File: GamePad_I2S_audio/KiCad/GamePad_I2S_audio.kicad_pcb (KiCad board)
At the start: 4 copper layers, 42.2 x 47.1 mm, 48 parts, among them J1 Conn_02x17_Odd_Even

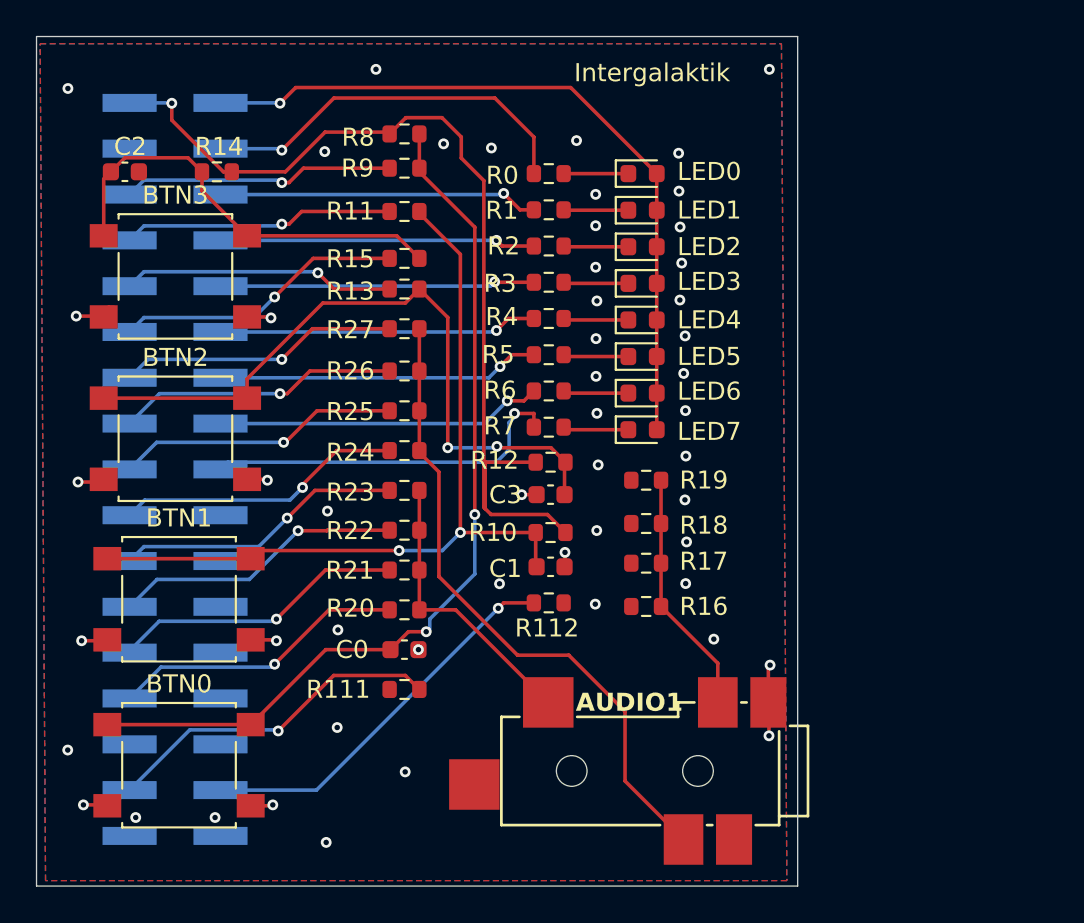
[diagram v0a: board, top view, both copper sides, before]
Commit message: initial PCB setup
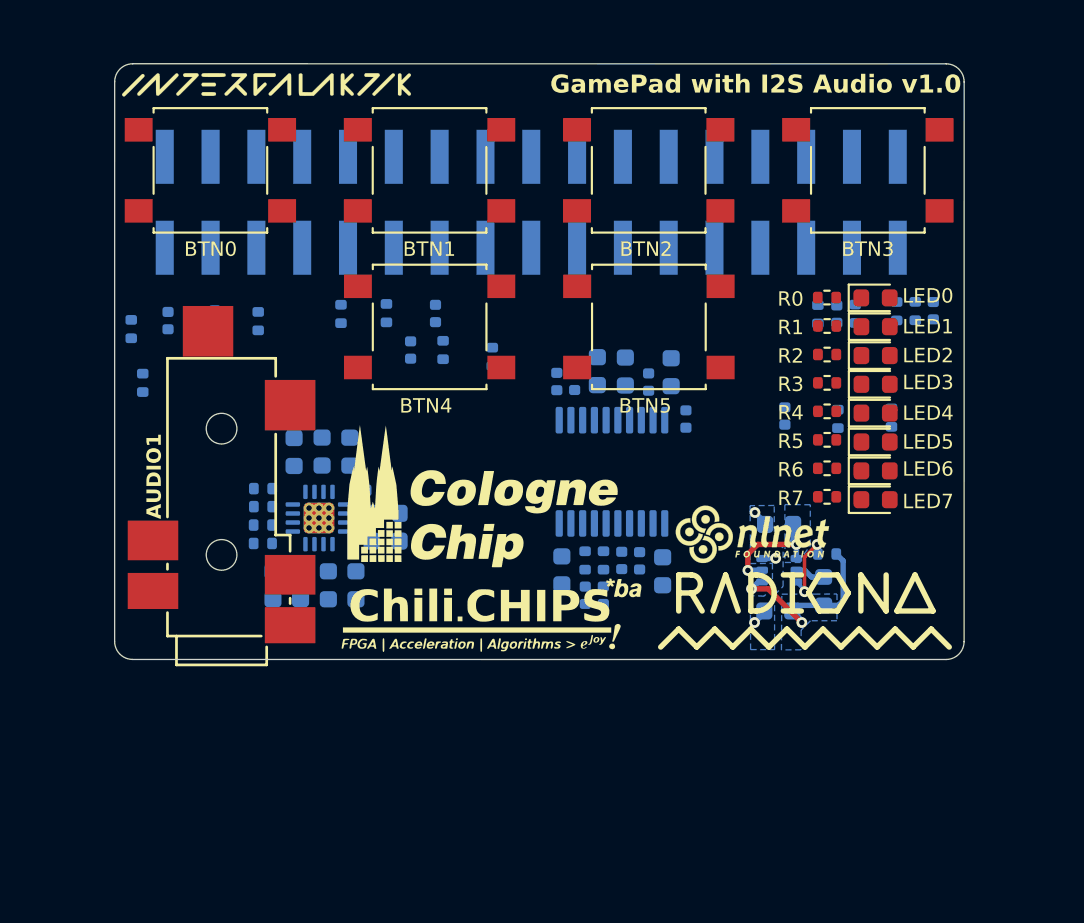
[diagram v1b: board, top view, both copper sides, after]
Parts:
- removed R21, R25: 549, Resistor_SMD:R_0603_1608Metric
- removed R22, R26: 270, Resistor_SMD:R_0603_1608Metric
- removed R23, R27: 130, Resistor_SMD:R_0603_1608Metric
- removed R24: 1.1k, Resistor_SMD:R_0603_1608Metric
- added BTN4: BTN, Button_Switch_SMD:SW_SPST_B3S-1000, F.Cu at (128.9, 68.7)
- added BTN5: BTN, Button_Switch_SMD:SW_SPST_B3S-1000, F.Cu at (141.1, 68.7)
- added C10: 100nF, Capacitor_SMD:C_0402_1005Metric, B.Cu at (141.0, 71.8)
- added C11: 10uF, Capacitor_SMD:C_0603_1608Metric, B.Cu at (138.2, 71.2)
- added C12: 2.2nF, Capacitor_SMD:C_0402_1005Metric, B.Cu at (138.5, 83.6)
- added C13: 10uF, Capacitor_SMD:C_0603_1608Metric, B.Cu at (139.7, 71.2)
- added C14: 100nF, Capacitor_SMD:C_0402_1005Metric, B.Cu at (135.9, 71.7)
- added C15: 10uF, Capacitor_SMD:C_0603_1608Metric, B.Cu at (142.3, 71.2)
- added C16: 100nF, Capacitor_SMD:C_0402_1005Metric, B.Cu at (143.1, 73.8)
- added C17: 4.7u, Capacitor_SMD:C_0603_1608Metric, B.Cu at (124.8, 83.0)
- added C18: 4.7u, Capacitor_SMD:C_0603_1608Metric, B.Cu at (123.3, 83.0)
- added C19: 4.7u, Capacitor_SMD:C_0603_1608Metric, B.Cu at (121.7, 83.0)
- added C20: 4.7u, Capacitor_SMD:C_0603_1608Metric, B.Cu at (120.2, 83.0)
- added C21: 4.7u, Capacitor_SMD:C_0603_1608Metric, B.Cu at (126.5, 80.6)
- added C22: 1u, Capacitor_SMD:C_0603_1608Metric, B.Cu at (121.4, 75.6)
- added C23: 1u, Capacitor_SMD:C_0603_1608Metric, B.Cu at (124.5, 75.6)
- added C24: 1u, Capacitor_SMD:C_0603_1608Metric, B.Cu at (122.9, 75.6)
- added C25: 100nF/10V/20%/X5R/C0402, Capacitor_SMD:C_0402_1005Metric, B.Cu at (114.4, 68.3)
- added C26: 100nF/10V/20%/X5R/C0402, Capacitor_SMD:C_0402_1005Metric, B.Cu at (148.6, 73.6)
- added C27: 10uF, Capacitor_SMD:C_0603_1608Metric, B.Cu at (148.2, 84.5)
- added C28: 10uF, Capacitor_SMD:C_0603_1608Metric, B.Cu at (148.3, 79.7)
- added C4: 10uF, Capacitor_SMD:C_0603_1608Metric, B.Cu at (141.8, 82.2)
- added C5: 10uF, Capacitor_SMD:C_0603_1608Metric, B.Cu at (136.2, 82.2)
- added C6: 100nF, Capacitor_SMD:C_0402_1005Metric, B.Cu at (136.9, 71.7)
- added C7: 2.2uF, Capacitor_SMD:C_0402_1005Metric, B.Cu at (140.5, 81.7)
- added C8: 2.2uF, Capacitor_SMD:C_0402_1005Metric, B.Cu at (139.5, 81.6)
- added C9: 2.2nF, Capacitor_SMD:C_0402_1005Metric, B.Cu at (137.5, 83.6)
- added G***: LOGO, nlnet:nlnet, F.Cu at (146.8, 80.2)
- added G***: LOGO, Cologne:cologne, F.Cu at (131.8, 78.1)
- added G***: LOGO, PCM_Intergalaktik:Intergalaktik logo, F.Cu at (119.9, 55.1)
- added G***: LOGO, ChiliChips:ChiliChipsBa, F.Cu at (132.4, 84.6)
- added IC1: PCM5100, Package_SO:TSSOP-20_4.4x6.5mm_P0.65mm, B.Cu at (139.0, 76.7)
- added IC2: PAM8908, Package_DFN_QFN:QFN-16-1EP_3x3mm_P0.5mm_EP1.7x1.7mm_ThermalVias, B.Cu at (122.8, 79.3)
- added IC3: TLV61225DC, Package_TO_SOT_SMD:SOT-363_SC-70-6, B.Cu at (148.3, 82.2)
- added L1: 80R@100M, Inductor_SMD:L_0603_1608Metric, B.Cu at (126.5, 79.0)
- added L2: 4.7uH, Inductor_SMD:L_0603_1608Metric, B.Cu at (150.7, 83.3)
- added R30: 470, Resistor_SMD:R_0402_1005Metric, B.Cu at (138.5, 81.6)
- added R31: 470, Resistor_SMD:R_0402_1005Metric, B.Cu at (137.5, 81.6)
- added R32: 33K, Resistor_SMD:R_0402_1005Metric, B.Cu at (125.9, 77.8)
- added R33: 330, Resistor_SMD:R_0402_1005Metric, B.Cu at (119.7, 78.7)
- added R34: 33K, Resistor_SMD:R_0402_1005Metric, B.Cu at (119.7, 77.7)
- added R35: 330, Resistor_SMD:R_0402_1005Metric, B.Cu at (119.7, 79.7)
- added R36: 33K, Resistor_SMD:R_0402_1005Metric, B.Cu at (119.7, 80.7)
- added radiona: radiona, radiona:radiona, F.Cu at (149.7, 83.5)
- C0, C1, C2, C3: footprint Capacitor_SMD:C_0603_1608Metric -> Capacitor_SMD:C_0402_1005Metric; moved to B.Cu
- R0, R1, R2, R3, R4, R5, R6, R7: footprint Resistor_SMD:R_0603_1608Metric -> Resistor_SMD:R_0402_1005Metric
- R10, R11, R111, R112, R12, R13, R14, R15, R8, R9: footprint Resistor_SMD:R_0603_1608Metric -> Resistor_SMD:R_0402_1005Metric; moved to B.Cu
- R16: value 1.1k -> 22R/R0402; footprint Resistor_SMD:R_0603_1608Metric -> Resistor_SMD:R_0402_1005Metric; moved to B.Cu
- R17: value 549 -> 22R/R0402; footprint Resistor_SMD:R_0603_1608Metric -> Resistor_SMD:R_0402_1005Metric; moved to B.Cu
- R18: value 270 -> 10K/R0402; footprint Resistor_SMD:R_0603_1608Metric -> Resistor_SMD:R_0402_1005Metric; moved to B.Cu
- R19: value 130 -> 10K/R0402; footprint Resistor_SMD:R_0603_1608Metric -> Resistor_SMD:R_0402_1005Metric; moved to B.Cu
- R20: value 1.1k -> 10K; footprint Resistor_SMD:R_0603_1608Metric -> Resistor_SMD:R_0402_1005Metric; moved to B.Cu
- moved BTN3 50.5 mm to (153.2, 60.0)
- moved BTN2 35.3 mm to (141.0, 60.0)
- moved C0 34.8 mm to (156.8, 67.8), turned to -90 degrees
- moved R8 30.0 mm to (155.8, 67.8), turned to 90 degrees
- moved R16 28.7 mm to (117.0, 68.3), turned to 90 degrees
- moved R9 28.4 mm to (154.8, 67.8), turned to -90 degrees
- moved AUDIO1 27.8 mm to (117.4, 78.3), turned to 180 degrees
- moved R112 25.6 mm to (113.0, 71.8), turned to 90 degrees
- moved R111 25.1 mm to (112.3, 68.8), turned to 90 degrees
- moved J1 24.7 mm to (134.5, 61.8), turned to 90 degrees
- moved R18 24.3 mm to (119.4, 68.4), turned to 90 degrees
- moved R20 23.6 mm to (150.9, 81.3)
- moved R11 23.6 mm to (150.4, 68.0), turned to -90 degrees
- moved C1 21.2 mm to (151.5, 68.0), turned to 90 degrees
- moved R10 20.8 mm to (152.5, 68.0), turned to 90 degrees
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- renumbered BTN3 to BTN0, BTN2 to BTN1, BTN1 to BTN2, BTN0 to BTN3
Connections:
- AUDIO1 pad 2: /AUDIO_L -> /HP_OUTL
- AUDIO1 pad 3: /AUDIO_R -> /HP_OUTR
- J1 pad 13: AUDIO_R3 -> /SB_B3
- J1 pad 15: AUDIO_R2 -> /SB_A3
- J1 pad 17: AUDIO_R1 -> AMP_EN
- J1 pad 19: AUDIO_R0 -> /SB_A2
- J1 pad 21: AUDIO_L3 -> I2S1_TX_WS
- J1 pad 23: AUDIO_L2 -> I2S1_TX_SDA
- J1 pad 25: AUDIO_L1 -> I2S1_TX_SCK
- J1 pad 27: AUDIO_L0 -> AUDIO_MUTE
- R16 pad 1: AUDIO_V0 -> /SB_B3
- R16 pad 2: /AUDIO_V -> Net-(BTN4-Pad1)
- R17 pad 1: AUDIO_V1 -> /SB_A3
- R17 pad 2: /AUDIO_V -> Net-(BTN5-Pad1)
- R18 pad 1: AUDIO_V2 -> Net-(BTN4-Pad1)
- R18 pad 2: /AUDIO_V -> +2V5
- R19 pad 1: AUDIO_V3 -> Net-(BTN5-Pad1)
- R19 pad 2: /AUDIO_V -> +2V5
- R20 pad 1: AUDIO_L0 -> /SB_A2
- R20 pad 2: /AUDIO_L -> +2V5
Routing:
- net Net-(BTN0-Pad1): track 49.8 -> 0.00 mm, vias 2 -> 0
- net Net-(BTN1-Pad1): track 45.1 -> 0.00 mm, vias 2 -> 0
- net +2V5: track 53.5 -> 11.0 mm, vias 1 -> 2
- net +1V8: track 40.8 -> 0.00 mm, vias 1 -> 0
- net Net-(BTN2-Pad1): track 38.8 -> 0.00 mm, vias 2 -> 0
- net /AUDIO_R: track 36.1 -> 0.00 mm
- net Net-(BTN3-Pad1): track 24.1 -> 0.00 mm
- net /WC_B3: track 21.8 -> 0.00 mm, vias 1 -> 0
- net Net-(J1-Pin_32): track 21.7 -> 0.00 mm, vias 1 -> 0
- net /WC_A0: track 20.4 -> 0.00 mm, vias 1 -> 0
- net Net-(J1-Pin_31): track 19.1 -> 0.00 mm, vias 1 -> 0
- net /WC_B0: track 18.1 -> 0.00 mm, vias 1 -> 0
- net /WC_A1: track 17.9 -> 0.00 mm, vias 1 -> 0
- net /WC_A3: track 17.8 -> 0.00 mm, vias 1 -> 0
- net /WC_B1: track 17.7 -> 0.00 mm, vias 1 -> 0
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- added copper zone on B.Cu, net +2V5
- added copper zone on B.Cu, net +3V3
- removed copper zone on F.Cu, net GND
- removed copper zone on In1.Cu, net GND
- removed copper zone on In2.Cu, net GND
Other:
- board size 42.2 x 47.1 mm -> 47.1 x 33 mm
- board text added: "2.5V>>3.3V"
- board text added: "AMP"
- board text added: "DAC"
- board text added: "GamePad with I2S Audio v1.0"
- board text removed: "Intergalaktik"
